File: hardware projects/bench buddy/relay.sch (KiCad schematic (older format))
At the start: 0 parts

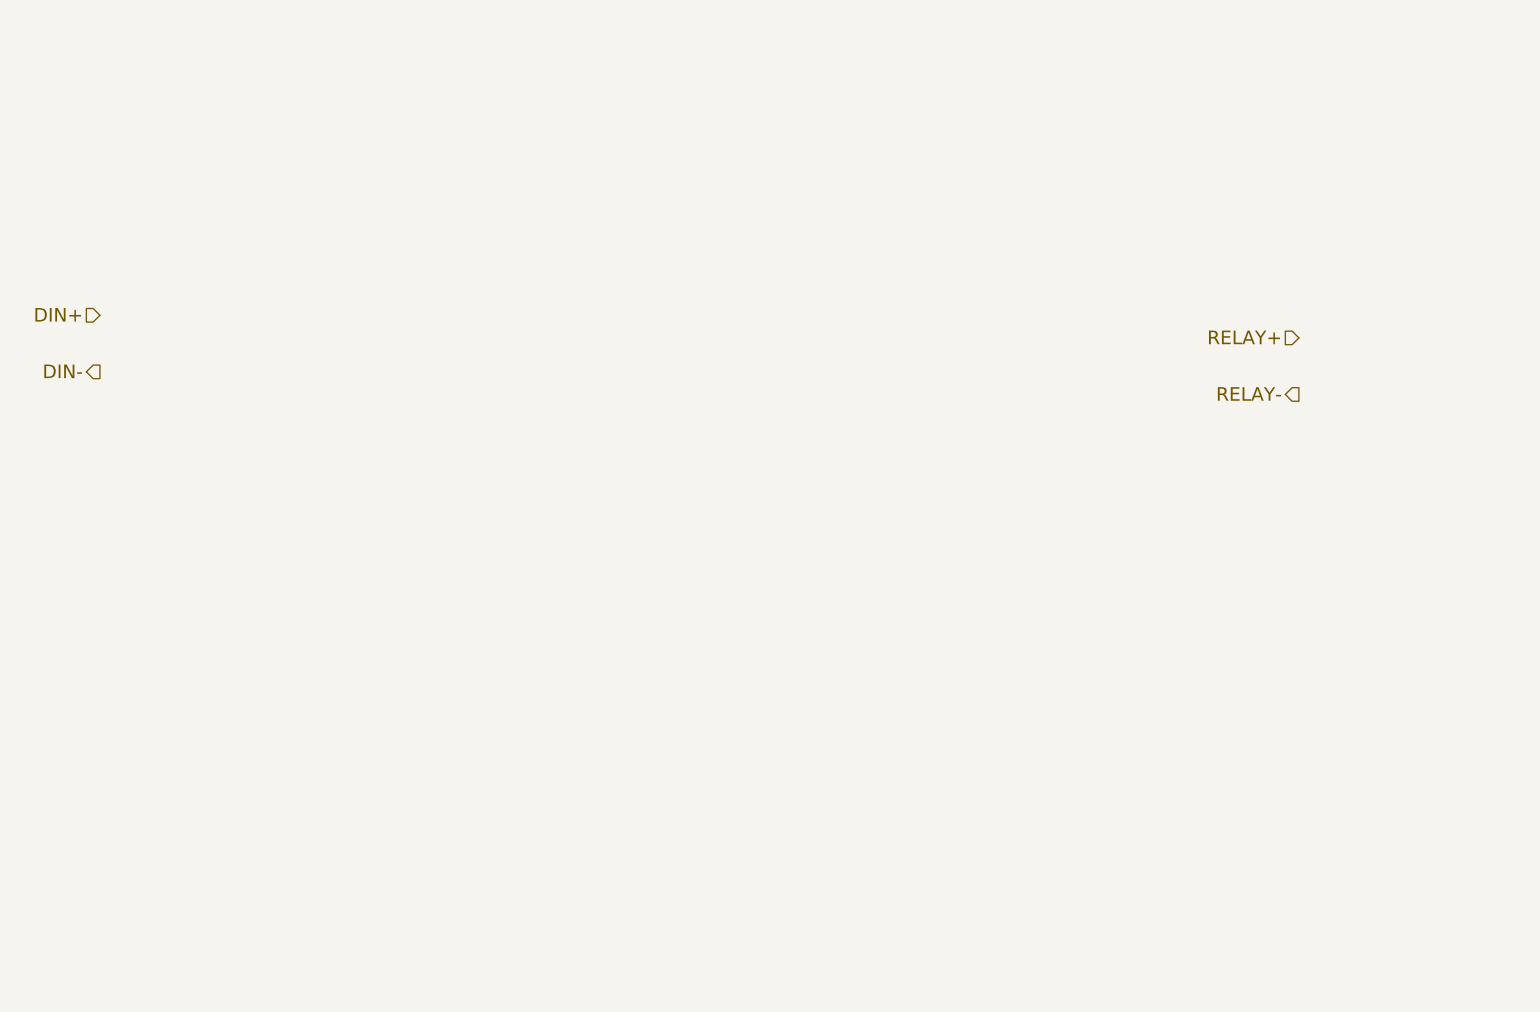
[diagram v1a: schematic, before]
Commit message: RELAY CONTROL
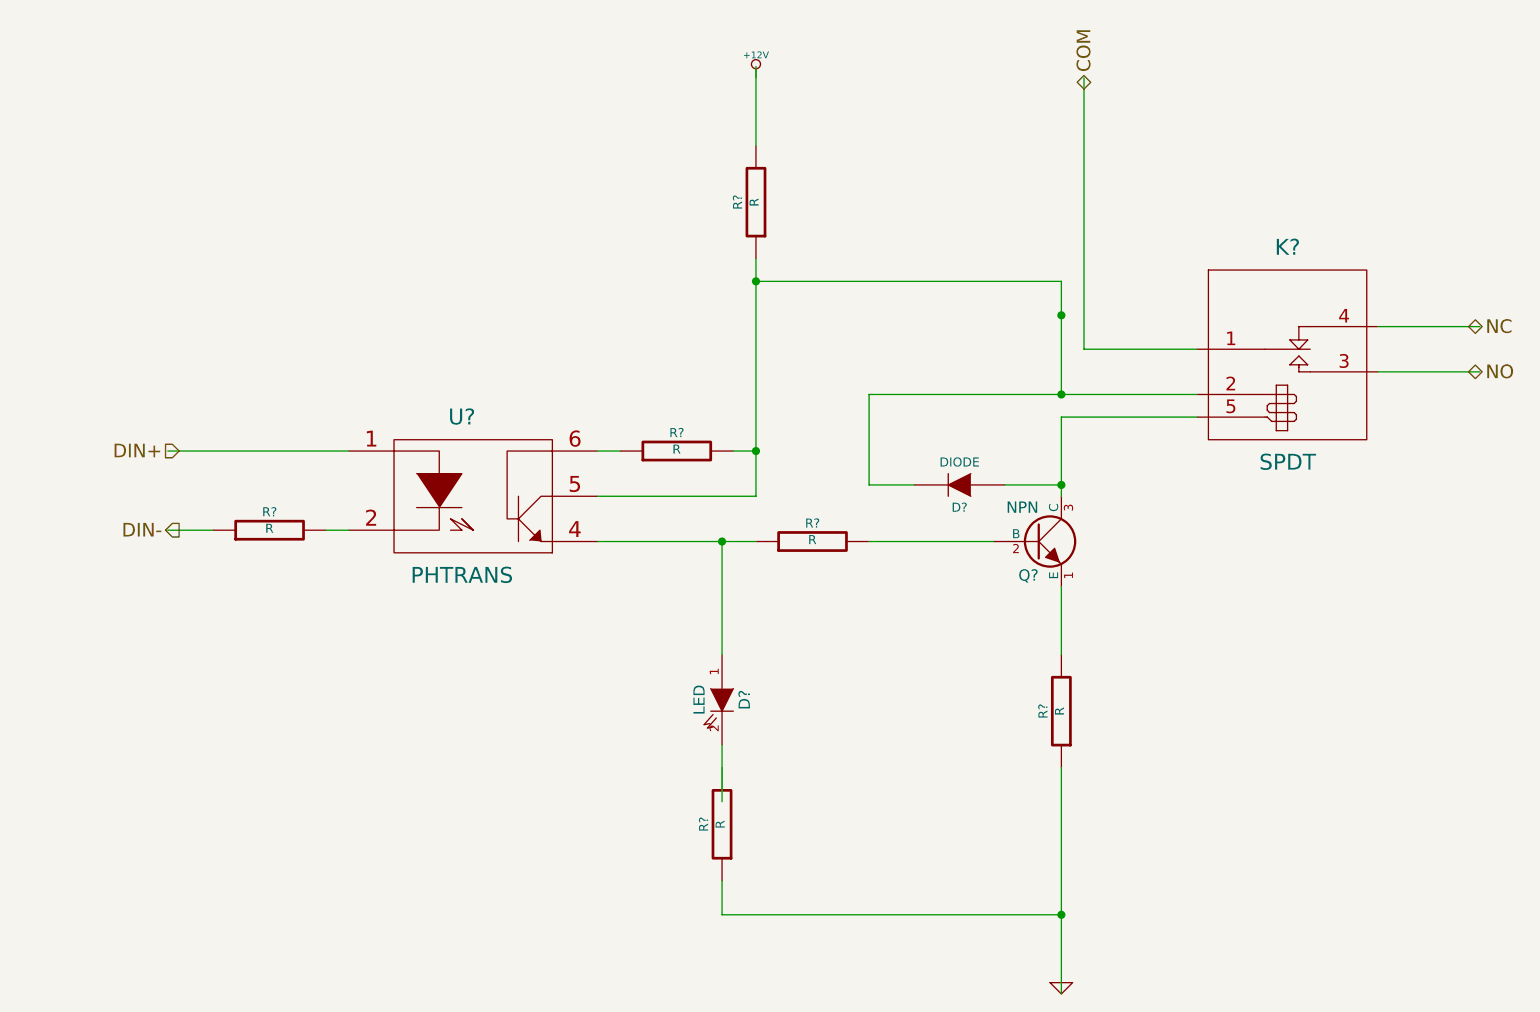
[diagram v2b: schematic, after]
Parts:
- added D?: LED, ~, symbol LED
- added D?: DIODE, ~, symbol DIODE
- added K?: SPDT, ~, symbol SPDT
- added Q?: NPN, ~, symbol NPN
- added R? (x6): R, ~, symbol R
- added U?: PHTRANS, ~, symbol PHTRANS
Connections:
- net labels added: +12V, COM, GND, NC, NO
- net labels removed: RELAY+, RELAY-
- wire segments 0 -> 28
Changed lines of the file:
@@
 LIBS:contrib
 LIBS:valves
+LIBS:BENCHBUDDEE
 LIBS:BenchBuddy-cache
 EELAYER 27 0
@@
 Sheet 4 8
 Title ""
-Date "13 mar 2015"
+Date "14 mar 2015"
 Rev ""
 Comp ""
@@
 Comment4 ""
 $EndDescr
-Text HLabel 8400 3650 0    60   Input ~ 0
-RELAY+
-Text HLabel 8400 3900 0    60   Output ~ 0
-RELAY-
-Text HLabel 3100 3550 0    60   Input ~ 0
+Text HLabel 9150 3600 2    60   BiDi ~ 0
+NC
+Text HLabel 9150 3800 2    60   BiDi ~ 0
+NO
+Text HLabel 3450 4150 0    60   Input ~ 0
 DIN+
-Text HLabel 3100 3800 0    60   Output ~ 0
+Text HLabel 3450 4500 0    60   Output ~ 0
 DIN-
+$Comp
+L PHTRANS U?
+U 1 1 5503C821
+P 4750 4350
+F 0 "U?" H 4700 4700 70  0000 C CNN
+F 1 "PHTRANS" H 4700 4000 70  0000 C CNN
+F 2 "~" H 4750 4350 60  0000 C CNN
+F 3 "~" H 4750 4350 60  0000 C CNN
+	1    4750 4350
+	1    0    0    -1
+$EndComp
+$Comp
+L R R?
+U 1 1 5503C83F
+P 6250 4550
+F 0 "R?" V 6330 4550 40  0000 C CNN
+F 1 "R" V 6257 4551 40  0000 C CNN
+F 2 "~" V 6180 4550 30  0000 C CNN
+F 3 "~" H 6250 4550 30  0000 C CNN
+	1    6250 4550
+	0    -1   -1   0
+$EndComp
+$Comp
+L NPN Q?
+U 1 1 5503C84E
+P 7250 4550
+F 0 "Q?" H 7250 4400 50  0000 R CNN
+F 1 "NPN" H 7250 4700 50  0000 R CNN
+F 2 "~" H 7250 4550 60  0000 C CNN
+F 3 "~" H 7250 4550 60  0000 C CNN
+	1    7250 4550
+	1    0    0    -1
+$EndComp
+$Comp
+L LED D?
+U 1 1 5503C85D
+P 5850 5250
+F 0 "D?" H 5850 5350 50  0000 C CNN
+F 1 "LED" H 5850 5150 50  0000 C CNN
+F 2 "~" H 5850 5250 60  0000 C CNN
+F 3 "~" H 5850 5250 60  0000 C CNN
+	1    5850 5250
+	0    1    1    0
+$EndComp
+$Comp
+L SPDT K?
+U 1 1 5503D173
+P 8350 3700
+F 0 "K?" H 8350 4150 70  0000 C CNN
+F 1 "SPDT" H 8350 3200 70  0000 C CNN
+F 2 "~" H 8350 3750 60  0000 C CNN
+F 3 "~" H 8350 3750 60  0000 C CNN
+	1    8350 3700
+	1    0    0    -1
+$EndComp
+Text HLabel 7450 2550 1    60   BiDi ~ 0
+COM
+Wire Wire Line
+	7450 3700 7950 3700
+Wire Wire Line
+	7450 2500 7450 3700
+Wire Wire Line
+	8750 3600 9200 3600
+Wire Wire Line
+	8750 3800 9200 3800
+Wire Wire Line
+	5300 4550 6000 4550
+Wire Wire Line
+	6500 4550 7050 4550
+$Comp
+L R R?
+U 1 1 5503D1DC
+P 5850 5800
+F 0 "R?" V 5930 5800 40  0000 C CNN
+F 1 "R" V 5857 5801 40  0000 C CNN
+F 2 "~" V 5780 5800 30  0000 C CNN
+F 3 "~" H 5850 5800 30  0000 C CNN
+	1    5850 5800
+	-1   0    0    1
+$EndComp
+$Comp
+L R R?
+U 1 1 5503D1E7
+P 7350 5300
+F 0 "R?" V 7430 5300 40  0000 C CNN
+F 1 "R" V 7357 5301 40  0000 C CNN
+F 2 "~" V 7280 5300 30  0000 C CNN
+F 3 "~" H 7350 5300 30  0000 C CNN
+	1    7350 5300
+	-1   0    0    1
+$EndComp
+$Comp
+L R R?
+U 1 1 5503D1ED
+P 6000 3050
+F 0 "R?" V 6080 3050 40  0000 C CNN
+F 1 "R" V 6007 3051 40  0000 C CNN
+F 2 "~" V 5930 3050 30  0000 C CNN
+F 3 "~" H 6000 3050 30  0000 C CNN
+	1    6000 3050
+	-1   0    0    1
+$EndComp
+$Comp
+L R R?
+U 1 1 5503D1F3
+P 3850 4500
+F 0 "R?" V 3930 4500 40  0000 C CNN
+F 1 "R" V 3857 4501 40  0000 C CNN
+F 2 "~" V 3780 4500 30  0000 C CNN
+F 3 "~" H 3850 4500 30  0000 C CNN
+	1    3850 4500
+	0    -1   -1   0
+$EndComp
+Wire Wire Line
+	7950 4000 7350 4000
+Wire Wire Line
+	7350 4000 7350 4350
+Wire Wire Line
+	7350 4750 7350 5050
+Wire Wire Line
+	5850 4550 5850 5050
+Connection ~ 5850 4550
+Wire Wire Line
+	5850 5450 5850 5700
+Wire Wire Line
+	5850 6200 7350 6200
+Wire Wire Line
+	7350 5550 7350 6550
+Connection ~ 7350 6200
+$Comp
+L GND #PWR?
+U 1 1 5503D252
+P 7350 6500
+F 0 "#PWR?" H 7350 6500 30  0001 C CNN
+F 1 "GND" H 7350 6430 30  0001 C CNN
+F 2 "" H 7350 6500 60  0000 C CNN
+F 3 "" H 7350 6500 60  0000 C CNN
+	1    7350 6500
+	1    0    0    -1
+$EndComp
+Wire Wire Line
+	5850 6050 5850 6200
+Wire Wire Line
+	6000 3300 6000 4350
+Wire Wire Line
+	6000 4350 5300 4350
+Wire Wire Line
+	4100 4500 4200 4500
+Wire Wire Line
+	4200 4150 3400 4150
+Wire Wire Line
+	3600 4500 3400 4500
+Connection ~ 6000 4150
+Wire Wire Line
+	6500 3900 7950 3900
+Wire Wire Line
+	7350 3400 6000 3400
+Connection ~ 6000 3400
+$Comp
+L +12V #PWR?
+U 1 1 5503D360
+P 6000 2500
+F 0 "#PWR?" H 6000 2450 20  0001 C CNN
+F 1 "+12V" H 6000 2600 30  0000 C CNN
+F 2 "" H 6000 2500 60  0000 C CNN
+F 3 "" H 6000 2500 60  0000 C CNN
+	1    6000 2500
+	1    0    0    -1
+$EndComp
+Wire Wire Line
+	6000 2800 6000 2450
+Connection ~ 7350 4300
+Wire Wire Line
+	7350 3900 7350 3400
+$Comp
+L DIODE D?
+U 1 1 5503D447
+P 6900 4300
+F 0 "D?" H 6900 4400 40  0000 C CNN
+F 1 "DIODE" H 6900 4200 40  0000 C CNN
+F 2 "~" H 6900 4300 60  0000 C CNN
+F 3 "~" H 6900 4300 60  0000 C CNN
+	1    6900 4300
+	-1   0    0    1
+$EndComp
+Connection ~ 7350 3550
+$Comp
+L R R?
+U 1 1 5503D494
+P 5650 4150
+F 0 "R?" V 5730 4150 40  0000 C CNN
+F 1 "R" V 5657 4151 40  0000 C CNN
+F 2 "~" V 5580 4150 30  0000 C CNN
+F 3 "~" H 5650 4150 30  0000 C CNN
+	1    5650 4150
+	0    -1   -1   0
+$EndComp
+Wire Wire Line
+	6000 4150 5900 4150
+Wire Wire Line
+	5400 4150 5300 4150
+Wire Wire Line
+	6500 4300 6500 3900
+Connection ~ 7350 3900
+Wire Wire Line
+	7350 4300 7100 4300
+Wire Wire Line
+	6700 4300 6500 4300
 $EndSCHEMATC
